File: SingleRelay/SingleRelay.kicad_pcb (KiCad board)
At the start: 2 copper layers, 2 parts, among them Q1 2N7002

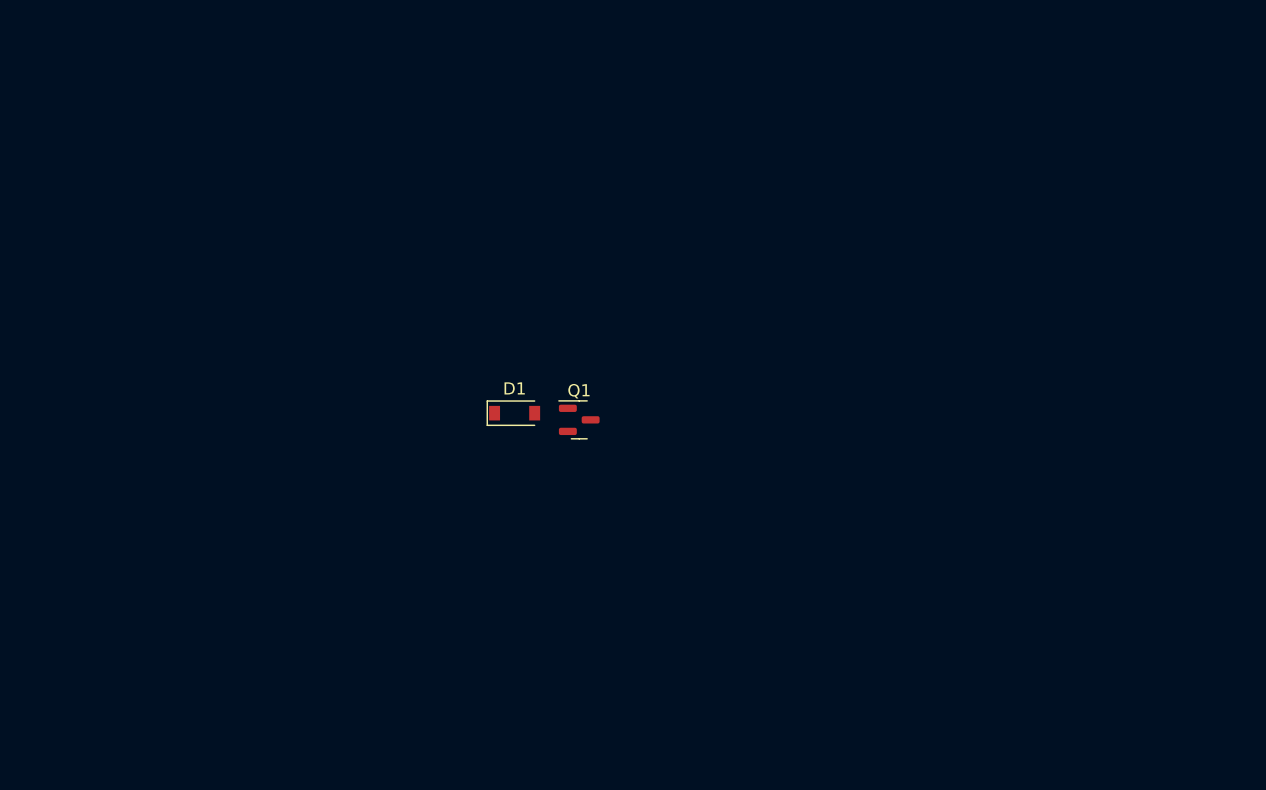
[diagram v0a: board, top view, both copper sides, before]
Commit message: 15:58 Arrakis.local
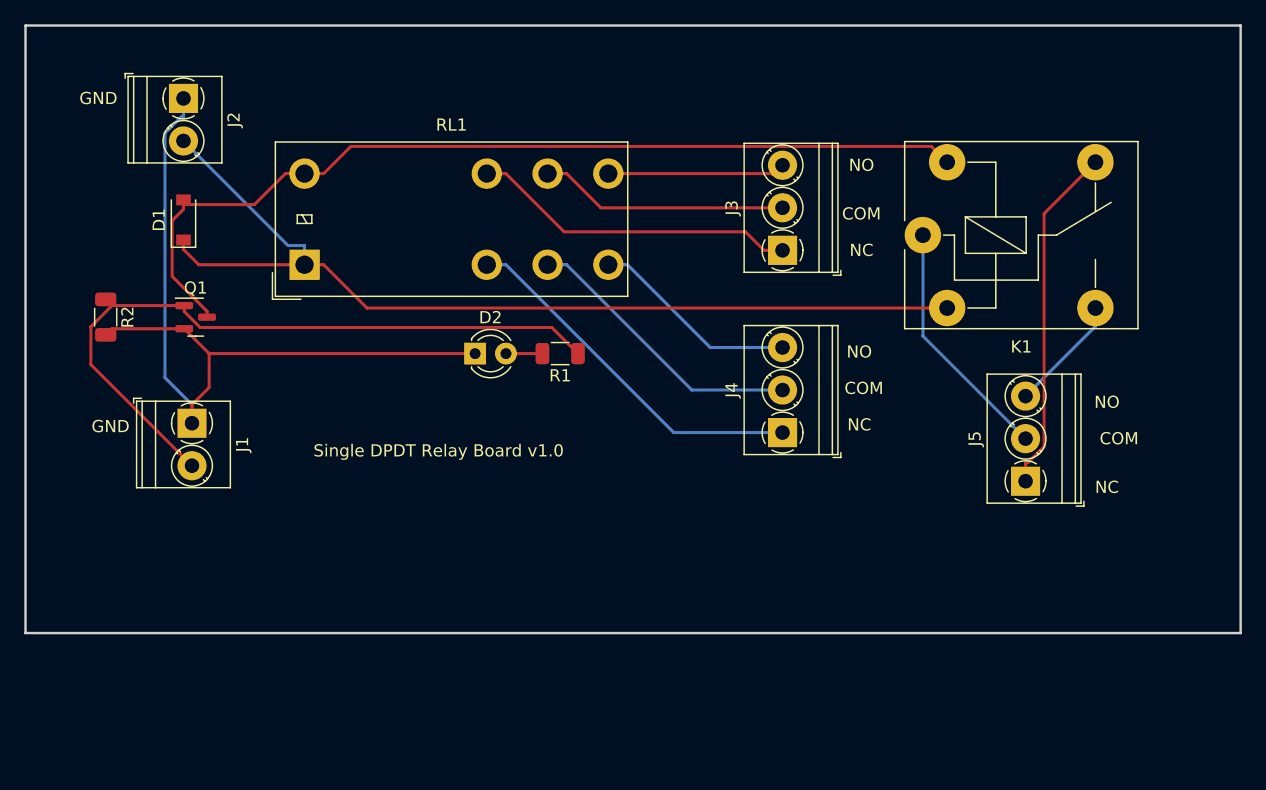
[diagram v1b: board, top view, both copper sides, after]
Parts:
- added D2: LED, LED_THT:LED_D3.0mm_Clear, F.Cu at (137.0, 77.0)
- added J1: Logic In, TerminalBlock_Phoenix:TerminalBlock_Phoenix_PT-1,5-2-3.5-H_1x02_P3.50mm_Horizontal, F.Cu at (113.7, 82.7)
- added J2: Relay Power, TerminalBlock_Phoenix:TerminalBlock_Phoenix_PT-1,5-2-3.5-H_1x02_P3.50mm_Horizontal, F.Cu at (113.0, 56.0)
- added J3: OUT1, TerminalBlock_Phoenix:TerminalBlock_Phoenix_PT-1,5-3-3.5-H_1x03_P3.50mm_Horizontal, F.Cu at (162.3, 68.5)
- added J4: OUT2, TerminalBlock_Phoenix:TerminalBlock_Phoenix_PT-1,5-3-3.5-H_1x03_P3.50mm_Horizontal, F.Cu at (162.3, 83.5)
- added J5: OUT3, TerminalBlock_Phoenix:TerminalBlock_Phoenix_PT-1,5-3-3.5-H_1x03_P3.50mm_Horizontal, F.Cu at (182.3, 87.5)
- added K1: FINDER-36.11, Relay_THT:Relay_SPDT_Finder_36.11, F.Cu at (173.8, 67.2)
- added R1: 10k, Resistor_SMD:R_1206_3216Metric, F.Cu at (144.0, 77.0)
- added R2: 10k, Resistor_SMD:R_1206_3216Metric, F.Cu at (106.6, 74.0)
- added RL1: G2RL-2-DC5, Relay_THT:Relay_DPDT_Omron_G2RL, F.Cu at (123.0, 69.7)
- moved Q1 32.7 mm to (114.0, 74.0)
- moved D1 31.6 mm to (113.0, 66.0), turned to 90 degrees
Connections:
- D1 pad 1: unconnected-(D1-Pad1) -> +5V
- D1 pad 2: unconnected-(D1-Pad2) -> Net-(D1-Pad2)
- Q1 pad 1: unconnected-(Q1-Pad1) -> Net-(J1-Pad2)
- Q1 pad 2: unconnected-(Q1-Pad2) -> GND
- Q1 pad 3: unconnected-(Q1-Pad3) -> Net-(D1-Pad2)
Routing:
- net +5V: track 0.00 -> 80.7 mm
- net Net-(D1-Pad2): track 0.00 -> 76.6 mm
- net GND: track 0.00 -> 66.2 mm
- net Net-(J1-Pad2): track 0.00 -> 58.3 mm
- net Net-(J4-Pad1): track 0.00 -> 30.1 mm
- net Net-(J5-Pad1): track 0.00 -> 28.7 mm
- net Net-(J3-Pad1): track 0.00 -> 27.0 mm
- net Net-(J4-Pad2): track 0.00 -> 23.6 mm
- net Net-(J3-Pad2): track 0.00 -> 20.5 mm
- net Net-(J5-Pad2): track 0.00 -> 20.3 mm
- net Net-(J4-Pad3): track 0.00 -> 17.2 mm
- net Net-(J3-Pad3): track 0.00 -> 14.6 mm
- net Net-(J5-Pad3): track 0.00 -> 9.63 mm
- net Net-(D2-Pad2): track 0.00 -> 3.00 mm
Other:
- board outline added: 100 x 50 mm
- board text added: "COM"
- board text added: "GND"
- board text added: "NC"
- board text added: "NO"
- board text added: "Single DPDT Relay Board v1.0"

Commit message: 19:58 Titan.local
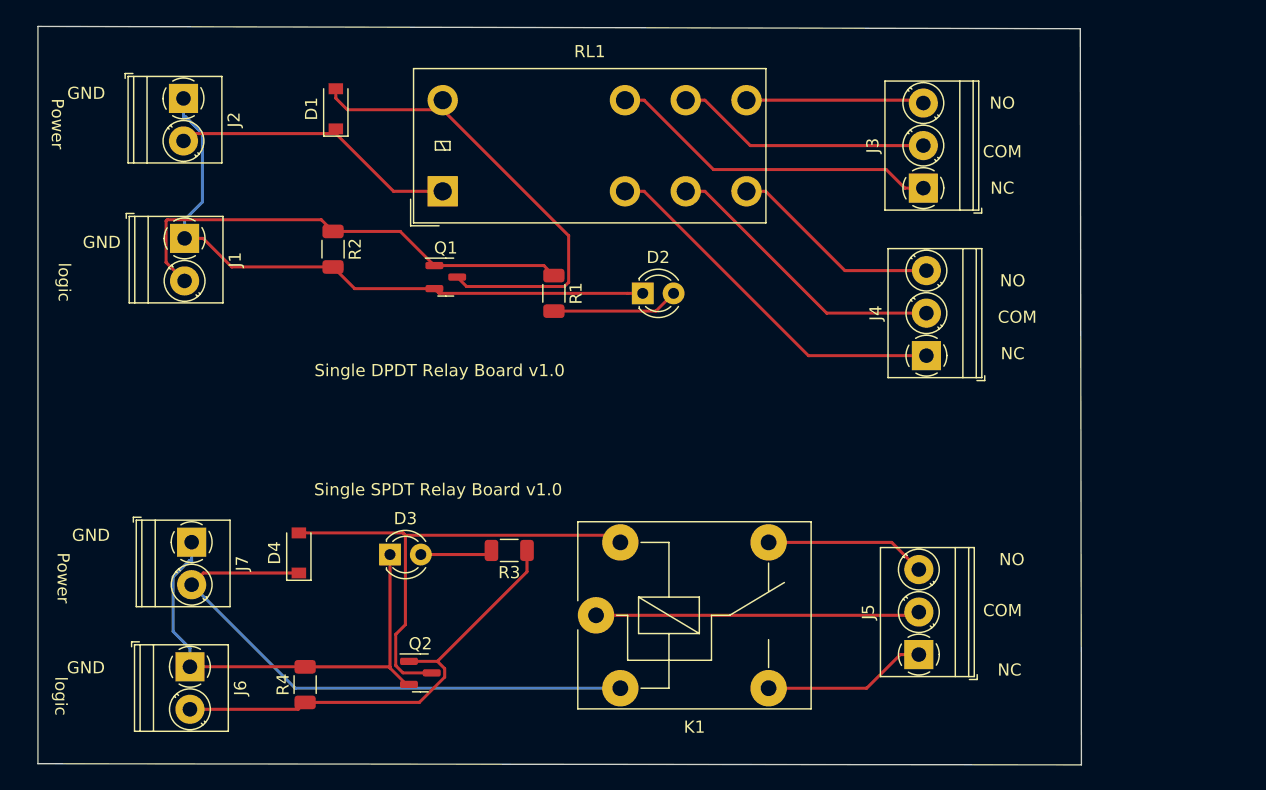
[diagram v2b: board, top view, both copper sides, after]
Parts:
- added D3: LED, LED_THT:LED_D3.0mm_Clear, F.Cu at (130.0, 93.5)
- added D4: 1N4148W, Diode_SMD:D_SOD-123, F.Cu at (122.5, 93.4)
- added J6: Logic In, TerminalBlock_Phoenix:TerminalBlock_Phoenix_PT-1,5-2-3.5-H_1x02_P3.50mm_Horizontal, F.Cu at (113.5, 102.8)
- added J7: Relay Power, TerminalBlock_Phoenix:TerminalBlock_Phoenix_PT-1,5-2-3.5-H_1x02_P3.50mm_Horizontal, F.Cu at (113.7, 92.5)
- added Q2: 2N7002, Package_TO_SOT_SMD:SOT-23, F.Cu at (132.5, 103.3)
- added R3: 10k, Resistor_SMD:R_1206_3216Metric, F.Cu at (139.8, 93.2)
- added R4: 10k, Resistor_SMD:R_1206_3216Metric, F.Cu at (123.0, 104.2)
- J5: value OUT3 -> OUT1
- moved K1 41.3 mm to (147.0, 98.5)
- moved Q1 20.8 mm to (134.6, 70.7)
- moved R2 19.5 mm to (125.3, 68.4)
- moved J5 16.8 mm to (173.5, 101.8)
- moved D1 15.5 mm to (125.5, 56.9)
- moved J1 15.2 mm to (113.1, 67.5)
- moved D2 14.7 mm to (150.8, 72.0)
- moved J4 13.4 mm to (174.1, 77.2)
- moved RL1 12.9 mm to (134.3, 63.6)
- moved J3 12.7 mm to (173.9, 63.4)
- moved R1 4.98 mm to (143.5, 72.0), turned to -90 degrees
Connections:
- K1 pad 12: Net-(J5-Pad1) -> Net-(J5-Pad3)
- K1 pad 14: Net-(J5-Pad3) -> Net-(J5-Pad1)
- K1 pad A1: +5V -> /5V
- K1 pad A2: Net-(D1-Pad2) -> Net-(K1-PadA2)
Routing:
- net +5V: track 80.7 -> 23.9 mm
- net /5V: track 0.00 -> 48.0 mm
- net Net-(K1-PadA2): track 0.00 -> 41.1 mm
- net /Gnd: track 0.00 -> 39.5 mm
- net Net-(J6-Pad2): track 0.00 -> 38.1 mm
- net Net-(D1-Pad2): track 76.6 -> 38.9 mm
- net Net-(J1-Pad2): track 58.3 -> 39.4 mm
- net Net-(J5-Pad1): track 28.7 -> 13.5 mm
- net GND: track 66.2 -> 52.5 mm
- net Net-(D2-Pad2): track 3.00 -> 10.5 mm
- net Net-(J5-Pad2): track 20.3 -> 26.7 mm
- net Net-(D3-Pad2): track 0.00 -> 5.95 mm
- net Net-(J5-Pad3): track 9.63 -> 13.3 mm
- net Net-(J3-Pad2): track 20.5 -> 21.1 mm
- net Net-(J3-Pad1): track 27.0 -> 27.6 mm
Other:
- board size 100 x 50 mm -> 85.9 x 60.8 mm
- board text added: "Power"
- board text added: "Single SPDT Relay Board v1.0"
- board text added: "logic"

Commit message: 20:04 Titan.local
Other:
- board text added: "V-Score"
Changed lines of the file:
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@@
     )
   )
+  (gr_line (start 101.106668 82.086749) (end 186.814425 82.086749) (layer "Dwgs.User") (width 2))
   (gr_line (start 186.897277 110.846591) (end 101.023818 110.752225) (layer "Edge.Cuts") (width 0.1))
   (gr_line (start 101.023818 50.074605) (end 186.80291 50.263338) (layer "Edge.Cuts") (width 0.1))
@@
     (effects (font (size 1 1) (thickness 0.15)))
   )
+  (gr_text "V-Score" (at 191.2146 81.799781) (layer "Dwgs.User")
+    (effects (font (size 1 1) (thickness 0.15)))
+  )
